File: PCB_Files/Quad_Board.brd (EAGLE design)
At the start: 83.5 x 78.7 mm, 47 parts, among them IC2 LM317MB, Q1 32.768kHz, Q2 KX-7 48MHz

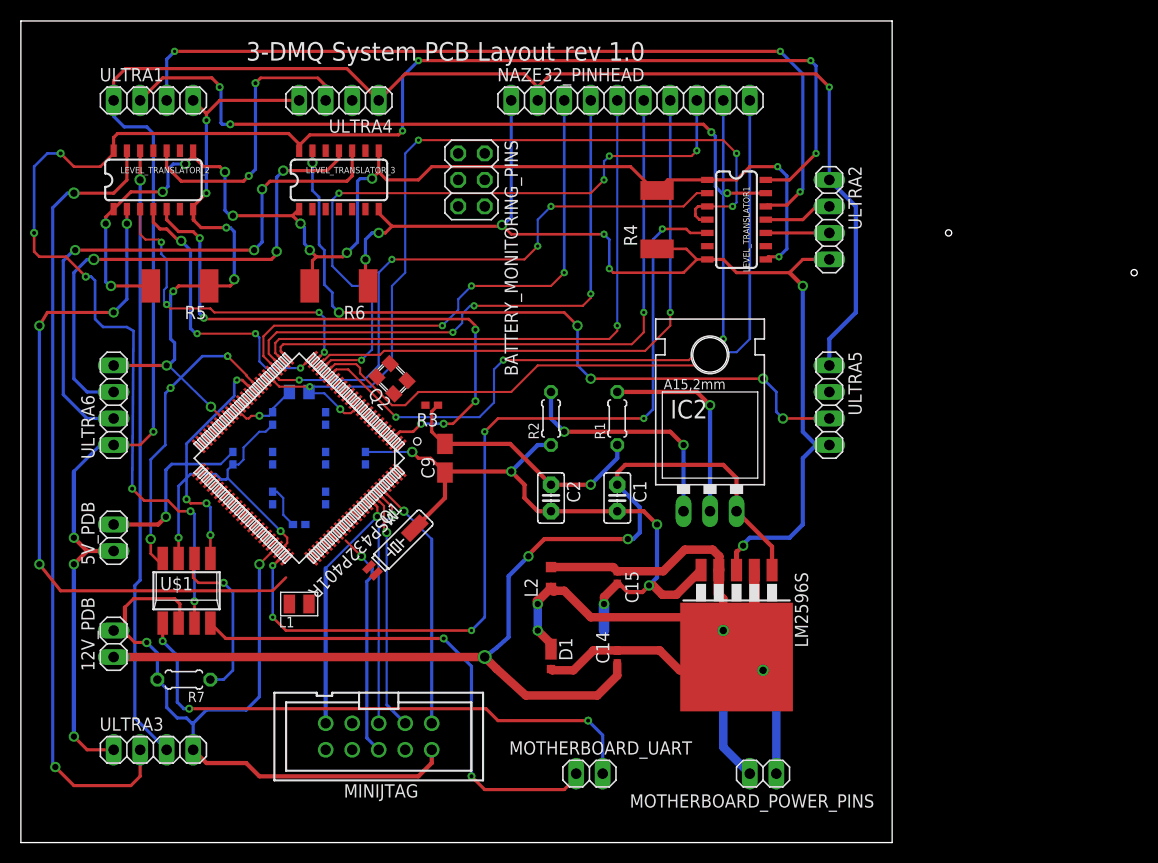
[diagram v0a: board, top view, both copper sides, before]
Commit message: Design Review PCB
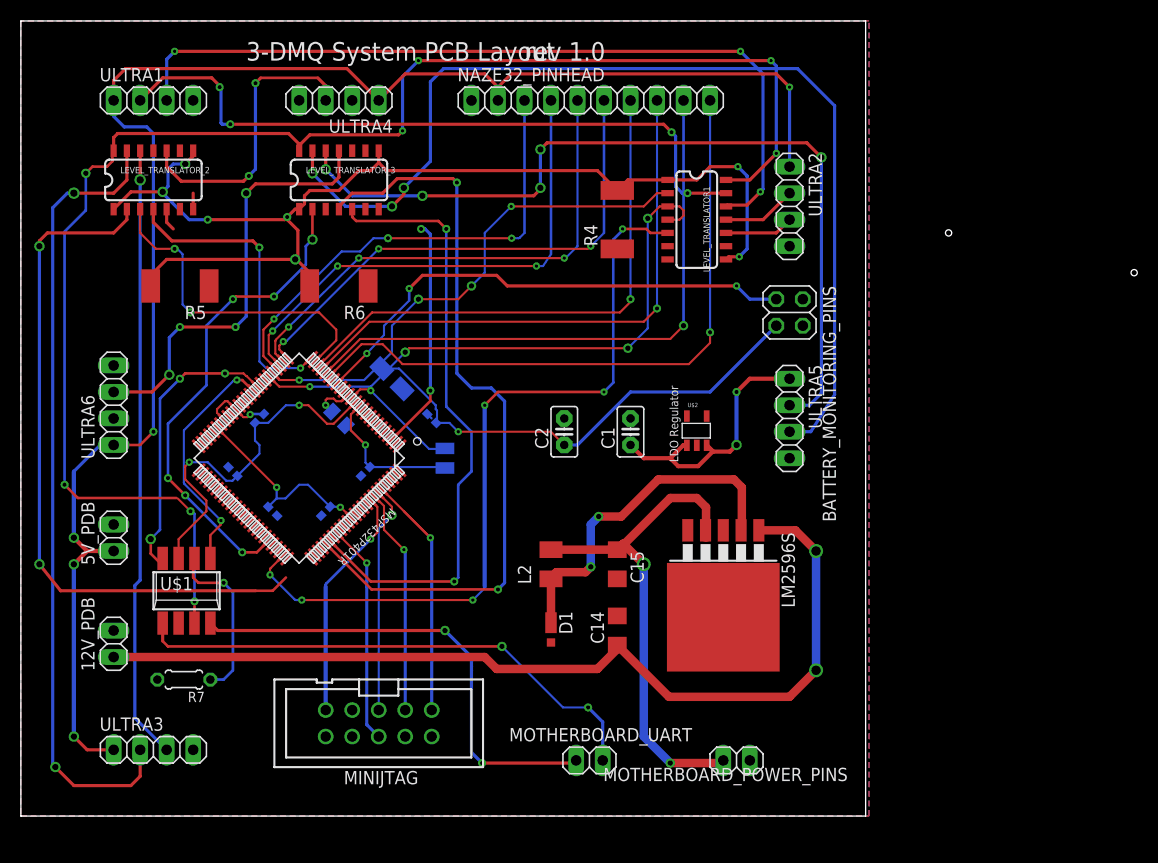
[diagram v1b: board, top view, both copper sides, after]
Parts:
- removed C12, C13: 22p, rcl:0402
- removed C5, C6: 12p, rcl:0402
- removed IC2: LM317MB, v-reg:TO220L1
- removed Q1: 32.768kHz, microcrystal:MS3V-T1R
- removed Q2: KX-7 48MHz, Geyer:KX-7
- removed R1, R2: (no value), rcl:0204/5
- added U$2: TLV733P, texas:SOT23-5
- BATTERY_MONITORING_PINS: device pinhead:2X03 -> pinhead:2X02
- C14, C15: device rcl:0402 -> eagle-ltspice:C1206
- L2: device resistor:L2012C -> resistor:L3225M
- moved BATTERY_MONITORING_PINS 33.0 mm to (73.7, 54.6)
- moved L1 19.8 mm to (40.6, 40.6), flipped to the bottom, turned to 90 degrees
- moved C9 9.16 mm to (35.6, 48.3), flipped to the bottom, turned to 45 degrees
- moved C1 6.48 mm to (58.4, 43.2), turned to 90 degrees
- moved C2 6.48 mm to (52.1, 43.2), turned to 90 degrees
- moved C3 5.24 mm to (29.2, 35.6), turned to 315 degrees
- moved C4 5.08 mm to (24.1, 35.6), turned to 225 degrees
- moved C11 4.58 mm to (33.0, 39.4), turned to 315 degrees
- moved C10 4.58 mm to (30.5, 44.5), turned to 45 degrees
- moved LM2596S 4.02 mm to (67.3, 27.9)
- moved ULTRA2 4.02 mm to (73.7, 64.8)
- moved ULTRA5 4.02 mm to (73.7, 44.5)
- moved LEVEL_TRANSLATOR1 3.81 mm to (64.8, 63.5)
- moved NAZE32_PINHEAD 3.81 mm to (54.6, 74.9)
- moved R4 3.81 mm to (57.1, 63.5)
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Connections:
- removed net N$28: IC2.1, R2.2
- removed net N$29: IC2.2, R1.2
- removed net N$7: C6.1, MSP432P401R.42, Q1.P1
- removed net N$8: C5.1, MSP432P401R.41, Q1.P2
- removed net P10.5_V: ULTRA4.2
- removed net P2.2/PM_UCA1RXD/PM_UCA1SOMI: MSP432P401R.18
- removed net P5.2/XT2IN1: C13.1, MSP432P401R.86, Q2.3
- removed net P5.3/XT2OUT1: C12.1, MSP432P401R.85, Q2.1
- new net PJ.0/LFXIN: MSP432P401R.41
- new net PJ.1/LFXOUT: MSP432P401R.42
- new net PJ.2/HFXOUT: MSP432P401R.85
- new net PJ.3/HFXIN: MSP432P401R.86
- net 12VDC: no longer C1.1, IC2.3
- net 3V3: now also BATTERY_MONITORING_PINS.3; no longer BATTERY_MONITORING_PINS.5, R1.1
- net 5VDC: now also C1.1, U$2.1, U$2.3
- net GND: now also BATTERY_MONITORING_PINS.4, U$2.2; no longer BATTERY_MONITORING_PINS.6, C12.2, C13.2, C5.2, C6.2, Q1.P3, R2.1
- net P10.5_5V: now also ULTRA4.2
- net P2.2_RX: now also MSP432P401R.18
- net P3.6_SDA: no longer BATTERY_MONITORING_PINS.3
- net P3.7_SCL: no longer BATTERY_MONITORING_PINS.4
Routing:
- net GND: track 369.8 -> 12.4 mm, vias 24 -> 2
- net P5.7_5V: track 0.00 -> 81.4 mm, vias 0 -> 5
- net P6.6: track 0.00 -> 73.4 mm, vias 0 -> 2
- net P6.7: track 0.00 -> 59.3 mm, vias 0 -> 2
- net P6.7_5V: track 55.0 -> 0.00 mm, vias 3 -> 0
- net P2.2_RX: track 0.00 -> 47.9 mm, vias 0 -> 3
- net P5.6: track 0.00 -> 46.8 mm, vias 0 -> 6
- net P10.3: track 55.7 -> 24.4 mm, vias 6 -> 2
- net P5.6_5V: track 71.1 -> 99.2 mm, vias 6 -> 3
- net 3V3: track 54.6 -> 81.5 mm
- net N$28: track 22.6 -> 0.00 mm, vias 2 -> 0
- net P8.1: track 77.5 -> 55.8 mm
- net N$2: track 0.00 -> 20.0 mm, vias 0 -> 2
- net N$29: track 19.6 -> 0.00 mm, vias 1 -> 0
- net 12VDC: track 104.0 -> 89.8 mm, vias 3 -> 2
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- added copper zone on layer 1, net GND
- added copper zone on layer 16, net GND
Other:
- board size 83.5 x 78.7 mm -> 81 x 76.2 mm
- board text added: "LDO Regulator"
